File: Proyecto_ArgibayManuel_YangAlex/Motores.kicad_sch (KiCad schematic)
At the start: 10 parts, among them K1 RT314012, K2 RT314012, Q1 2N2222, Q2 2N2222, U2 DRV8871DDA, U3 DRV8871DDA

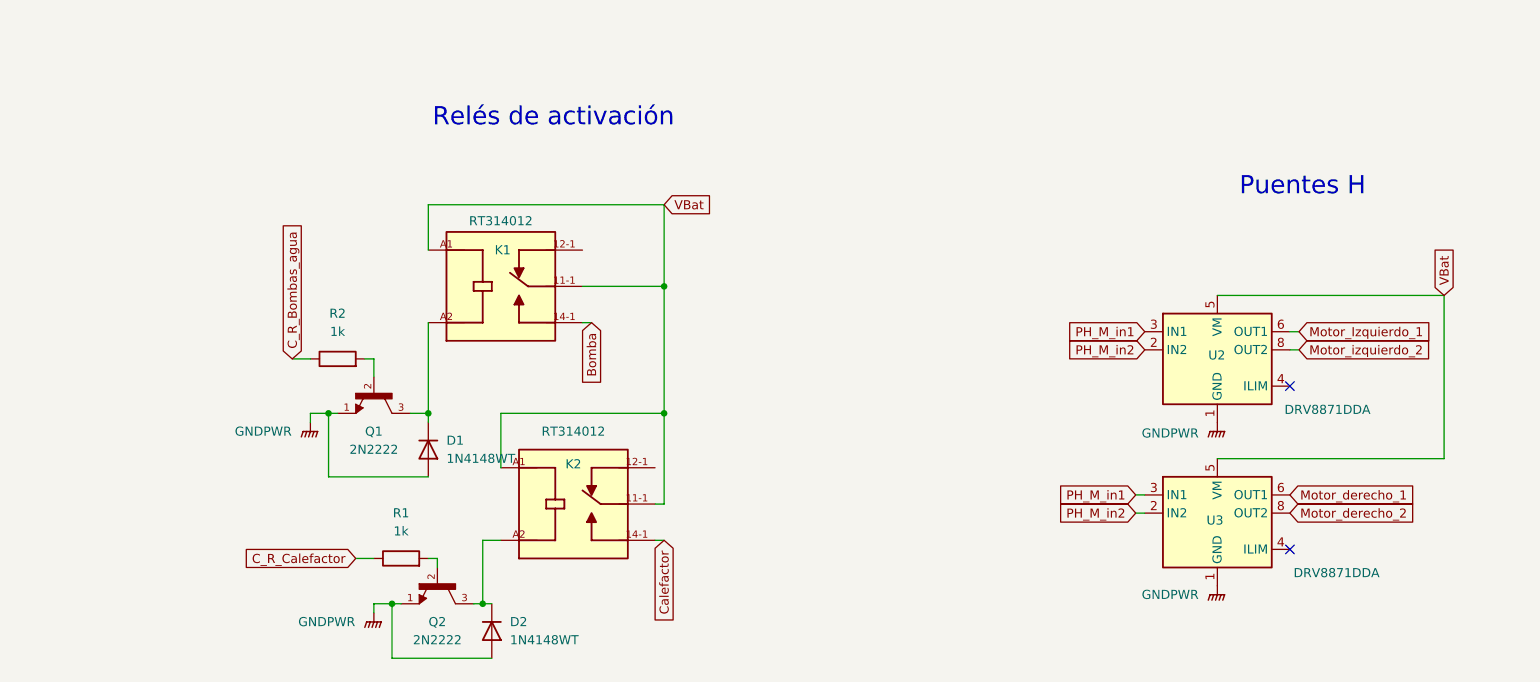
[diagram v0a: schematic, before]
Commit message: Ordenar esquematico
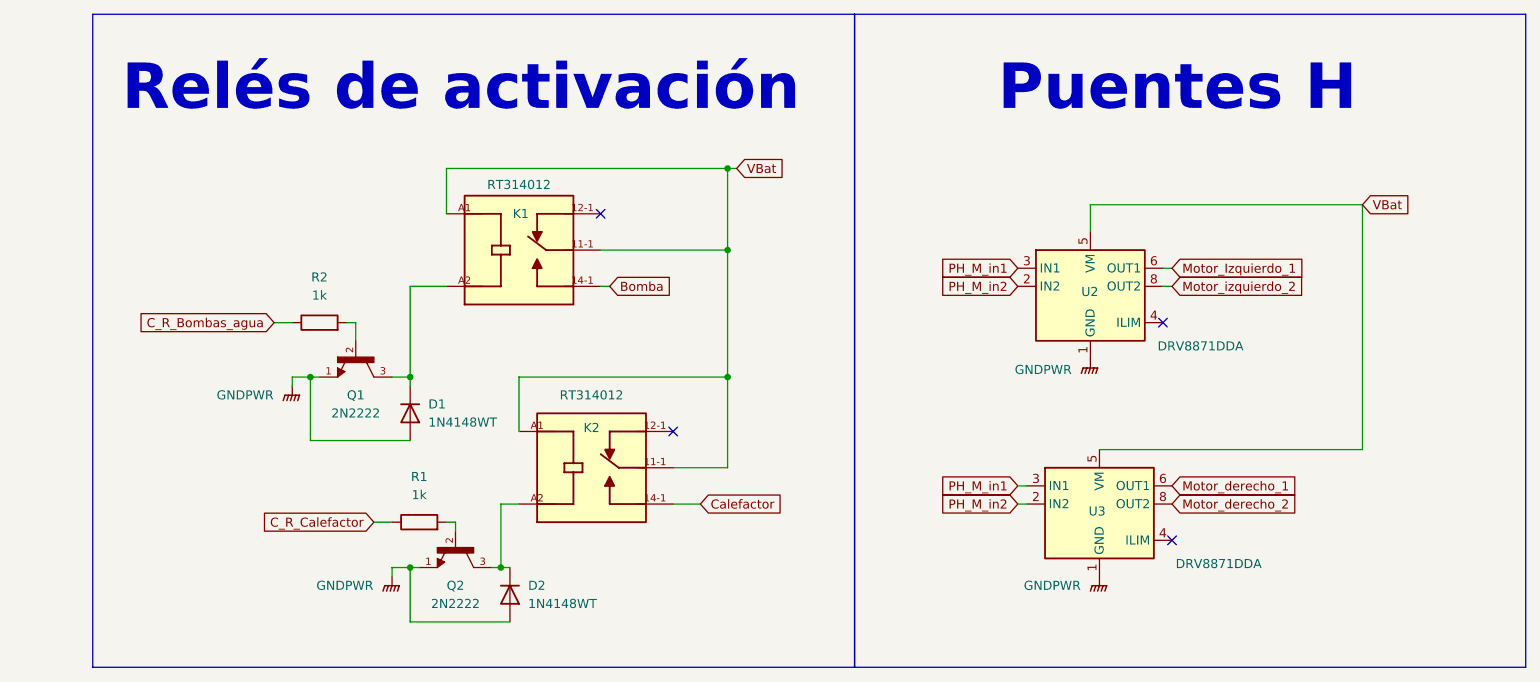
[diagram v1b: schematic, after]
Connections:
- no-connect marks 2 -> 4
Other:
- moved on the sheet: D1, D2, K1, K2, Q1, Q2, R1, R2, U2, U3
